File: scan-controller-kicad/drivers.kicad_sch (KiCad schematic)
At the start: 40 parts, among them CN4 Lamp, CN5 Fan, CN6 Motor, Q1 IRF7470, Q5 SS8050, U5 DRV8871DDA, U6 78L05, U7 XL4015, U8 TL431, U9 LM358

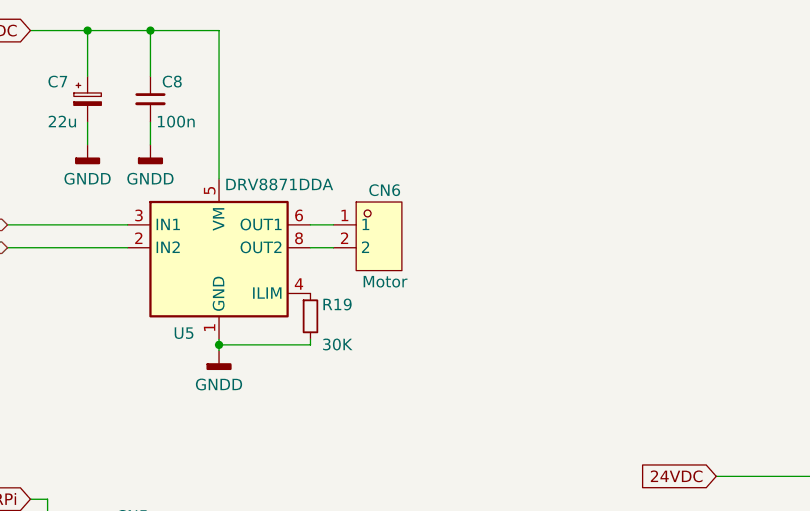
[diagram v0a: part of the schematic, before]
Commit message: Pushbutton PTHs now mechanical (DRC fun)
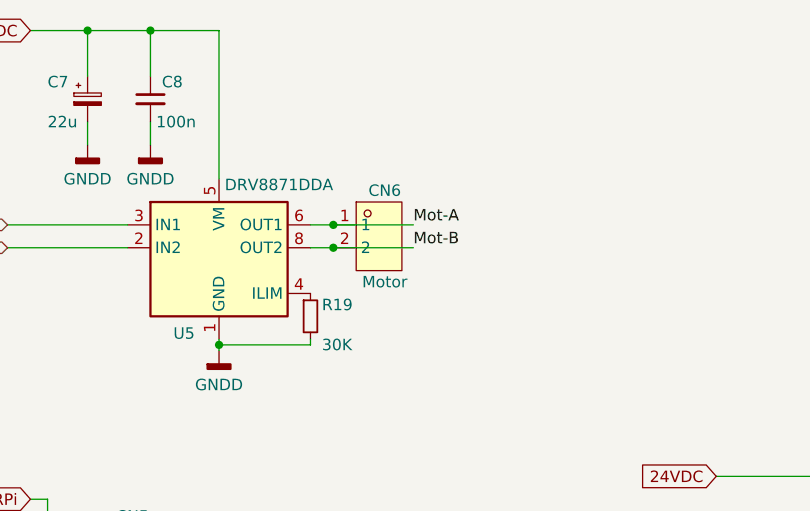
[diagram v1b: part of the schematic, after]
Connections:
- net Mot-A: now reaches CN6.1, U5.6 (OUT1)
- net Mot-B: now reaches CN6.2, U5.8 (OUT2)
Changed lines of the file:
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@@
 (kicad_sch (version 20230121) (generator eeschema)
   (paper "A4")
+  (junction (at 81.28 54.61) (diameter 0) (color 0 0 0 0)
+  )
   (junction (at 215.9 121.285) (diameter 0) (color 0 0 0 0)
   )
@@
   )
   (junction (at 201.93 92.71) (diameter 0) (color 0 0 0 0)
+  )
+  (junction (at 81.28 52.07) (diameter 0) (color 0 0 0 0)
   )
   (junction (at 169.545 121.285) (diameter 0) (color 0 0 0 0)
@@
     (stroke (width 0) (type default))
   )
+  (wire (pts (xy 81.28 52.07) (xy 90.17 52.07))
+    (stroke (width 0) (type default))
+  )
   (wire (pts (xy 165.735 119.38) (xy 165.735 121.285))
     (stroke (width 0) (type default))
@@
   )
   (wire (pts (xy 121.285 121.285) (xy 118.745 121.285))
+    (stroke (width 0) (type default))
+  )
+  (wire (pts (xy 81.28 54.61) (xy 90.17 54.61))
     (stroke (width 0) (type default))
   )
@@
     (effects (font (size 1.27 1.27)) (justify left bottom))
   )
+  (label "Mot-B" (at 90.17 54.61 0) (fields_autoplaced)
+    (effects (font (size 1.27 1.27)) (justify left bottom))
+  )
+  (label "Mot-A" (at 90.17 52.07 0) (fields_autoplaced)
+    (effects (font (size 1.27 1.27)) (justify left bottom))
+  )
